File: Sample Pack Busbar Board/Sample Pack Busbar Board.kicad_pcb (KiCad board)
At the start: 2 copper layers, 89.9 x 64.5 mm, 7 parts, among them J2 Conn_01x09_MountingPin

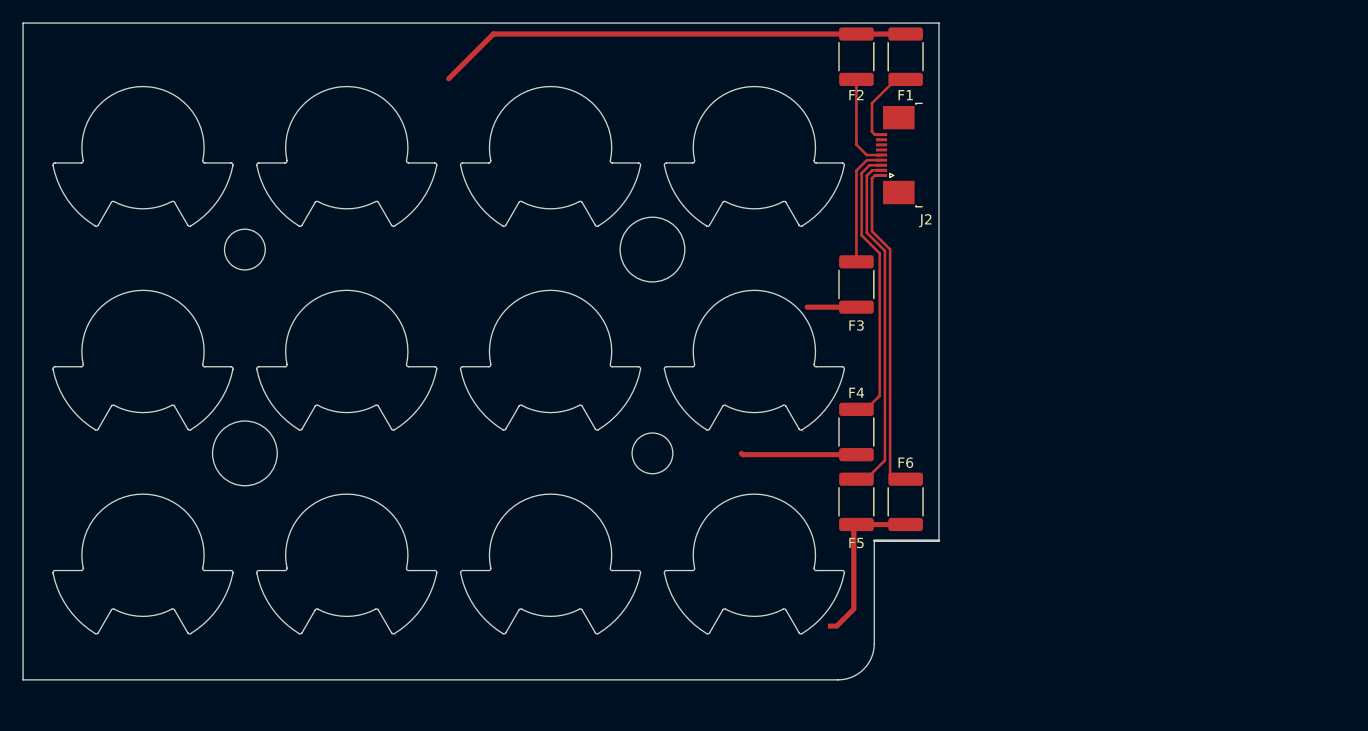
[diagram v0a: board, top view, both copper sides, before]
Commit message: changes for order
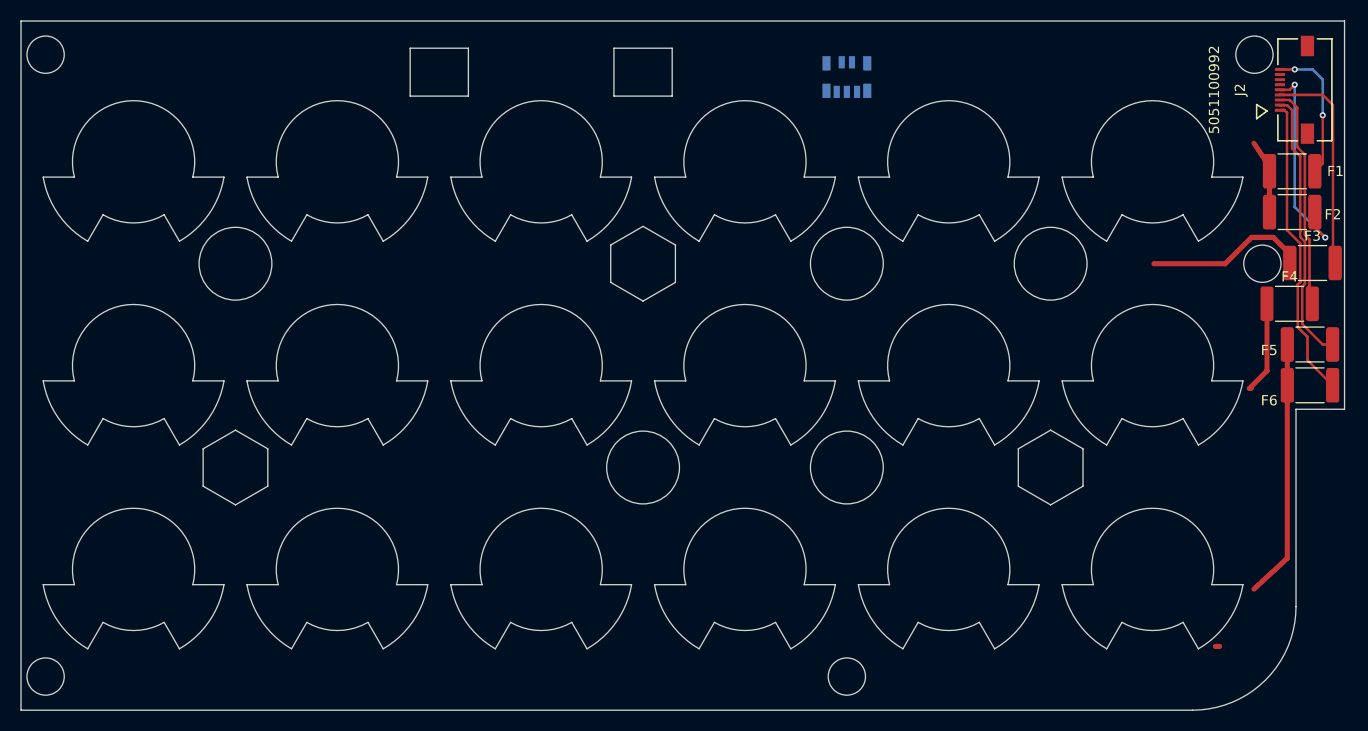
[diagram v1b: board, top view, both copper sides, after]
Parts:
- removed the J2 at (98.3, 25.7)
- added J2: Conn_01x09_MountingPin, FS_4_Global_Footprint_Library:CON_5051100992_MOL, F.Cu at (138.5, 19.2)
- added J2: 5019510550, formula_slug_footprint_library:CON_5019510550, B.Cu at (93.5, 18.0)
- moved F5 47.1 mm to (139.0, 44.2), turned to 0 degrees
- moved F2 45.4 mm to (137.2, 31.2), turned to 0 degrees
- moved F3 44.8 mm to (139.2, 36.2), turned to 0 degrees
- moved F4 44.3 mm to (137.0, 40.2), turned to 0 degrees
- moved F6 41.3 mm to (139.0, 48.2), turned to 0 degrees
- moved F1 39.6 mm to (137.2, 27.2), turned to 0 degrees
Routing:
- net /cell_2_plus: track 46.7 -> 4.00 mm
- net /cell_0_minus: track 4.83 -> 21.4 mm
- net /v_sense_cell_2: track 9.29 -> 20.8 mm, vias 0 -> 2
- net /cell_1_plus: track 4.84 -> 16.0 mm
- net /v_sense_cell_1: track 11.8 -> 21.2 mm
- net /v_sense_minus: track 33.9 -> 26.8 mm
- net /V+: track 8.12 -> 13.9 mm, vias 0 -> 2
- net /v_sense_cell_0: track 27.7 -> 22.0 mm
- net /V-: track 32.8 -> 29.6 mm
- net /cell_0_plus: track 11.3 -> 9.18 mm
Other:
- board size 89.9 x 64.5 mm -> 129.9 x 67.6 mm
